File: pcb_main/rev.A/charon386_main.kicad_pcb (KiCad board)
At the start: 4 copper layers, 100 x 100 mm, 143 parts, among them CON1 CF-CARD-cfcard, J1 Mini-DIN-6, J10 COM2, J11 ESP, J12 Conn_02x07_Odd_Even, J2 PJ-322, J3 USB_B_Micro, J4 Mini-DIN-6, J5 DB15_Female_HighDensity_Mount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, J6 Conn_01x04, J7 PC104_16, J8 PC104, J9 COM1, Q1 BC817, Q2 BC856, SW1 SW_Push, SW2 Jumper / Pin header 1x2 Pitch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, U1 CH340G, U10 LT1930, U11 TXB0104PW, U12 MAX823LEUK, U13 ST16C554, U14 74HCT32, U15 74HCT138, U16 74HCT138, U2 ESP-12E, U3 MSM5118160F-JS, U4 MSM5118160F-JS, U5 M6117D, U6 GD75232PW, U7 27C512PLCC, U8 GD75232PW, U9 AMS1117-3.3, X1 14.318 MHz, X3 80 MHz, Y1 12 MHz, Y2 32768 Hz, Y3 14.7456 MHz

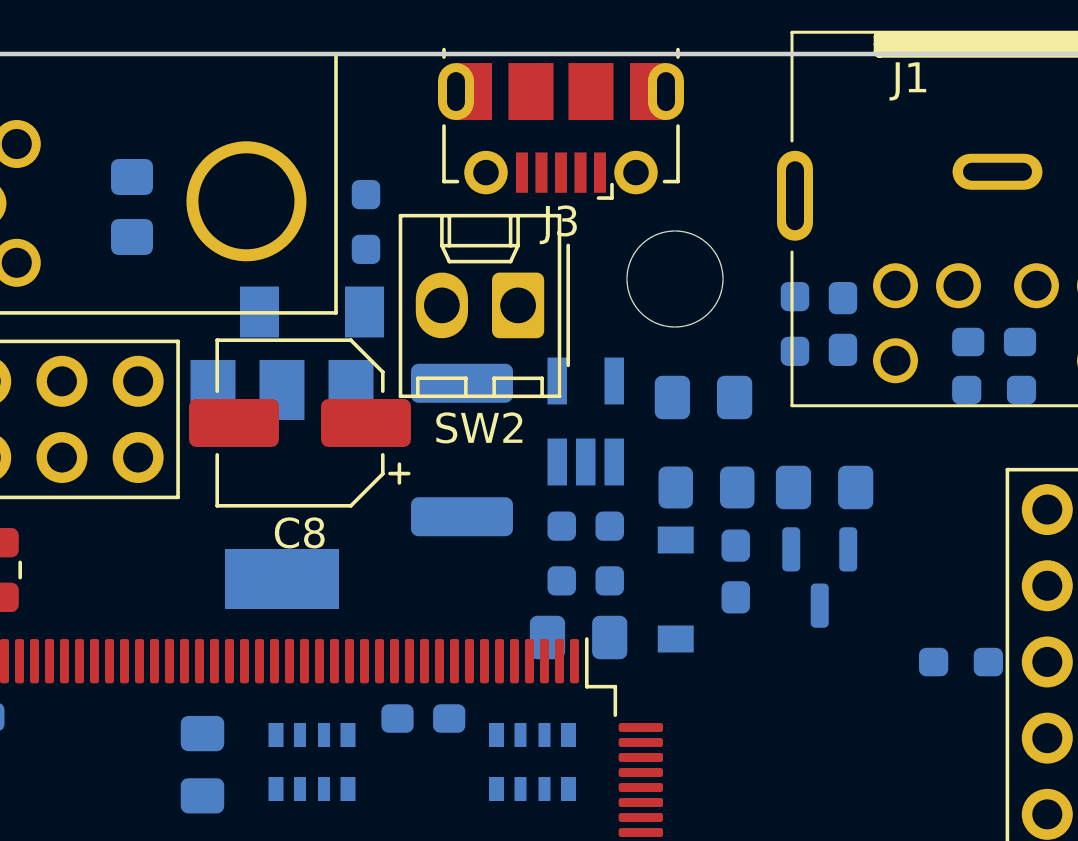
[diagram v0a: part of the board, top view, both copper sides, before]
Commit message: wip pcb rev.A
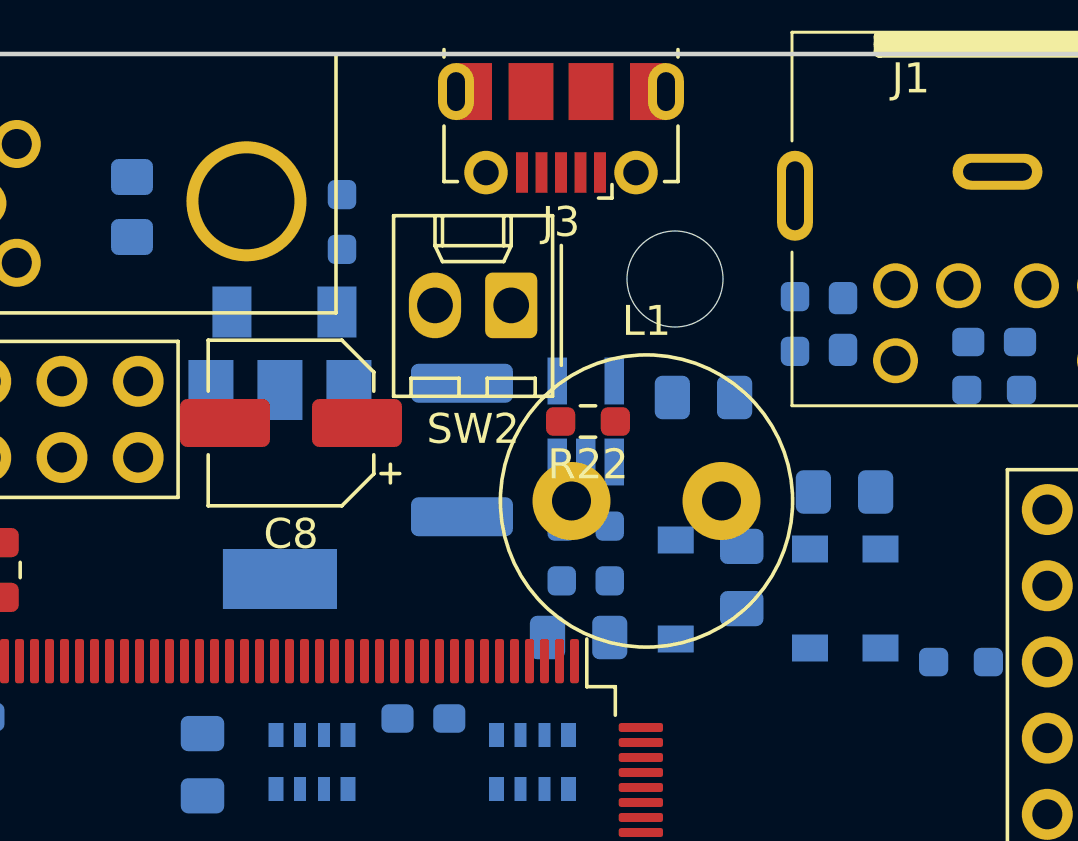
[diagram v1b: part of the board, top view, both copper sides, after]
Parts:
- added D9: MBR0520, Diode_SMD:D_SOD-123, B.Cu at (181.4, 65.8)
- added R22: 51k, Resistor_SMD:R_0603_1608Metric_Pad0.98x0.95mm_HandSolder, F.Cu at (174.0, 59.9)
- C15: footprint Capacitor_SMD:C_0603_1608Metric_Pad1.08x0.95mm_HandSolder -> Capacitor_SMD:C_0805_2012Metric_Pad1.18x1.45mm_HandSolder
- D4: value BAT54S -> MBR0520; footprint Package_TO_SOT_SMD:SOT-23 -> Diode_SMD:D_SOD-123
- L1: value L -> 10u; footprint Inductor_SMD:L_0805_2012Metric_Pad1.15x1.40mm_HandSolder -> Inductor_THT:L_Radial_D9.5mm_P5.00mm_Fastron_07HVP; moved to F.Cu
- R14: value R -> 113k
- R15: value R -> 13.3k
- moved L1 4.52 mm to (173.4, 62.5), turned to 0 degrees
- moved D4 2.14 mm to (183.8, 65.8)
- moved D7 0.92 mm to (163.9, 56.2)
- moved R21 0.80 mm to (165.8, 53.2)
- moved C16 0.68 mm to (182.6, 62.2)
- moved C8 0.30 mm to (164.1, 59.9)
- moved C15 0.28 mm to (179.1, 65.1)
- moved SW2 0.23 mm to (171.4, 56.0)
- moved D8 0.07 mm to (163.7, 62.0)
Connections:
- C57 pad 1: (no net) -> Net-(C57-Pad1)
- C58 pad 1: (no net) -> Net-(C58-Pad1)
- D4 pad 1: -12V -> GND
- D4 pad 2: GND -> Net-(C15-Pad2)
- J12 pad 15: unconnected-(J12-Pad15) -> (no net)
- U10 pad 4: +5V -> Net-(U10-Pad4)
- U13 pad 25: (no net) -> Net-(C57-Pad1)
- U13 pad 26: (no net) -> Net-(C58-Pad1)
- U14 pad 4: (no net) -> GND
- U14 pad 5: (no net) -> GND
- Y3 pad 1: (no net) -> Net-(C58-Pad1)
- Y3 pad 3: (no net) -> Net-(C57-Pad1)
